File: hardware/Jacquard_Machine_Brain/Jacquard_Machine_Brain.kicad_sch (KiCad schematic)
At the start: 69 parts, among them J1 Terminal Block, J15 USB_A, J16 Wurth_RJ45_LED, J2 Conn_01x08, J3 JST-SH 01x04, J4 Conn_01x02, J5 Conn_01x02, SW1 SW_DIP_x02, SW2 SW_MEC_5G, U1 R-78E5.0-1.0, U10 74AHCT1G125, U2 Teensy4.1, U3 74AHCT1G125, U4 74AHCT1G125, U5 74AHCT125, U6 AO4882, U7 74AHCT1G125, U8 74AHCT1G125, U9 PCA9306D

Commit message: sync
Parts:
- removed C6: 0.1uF, Capacitor_SMD:C_0402_1005Metric, symbol Device:C_Small
- removed JP1, JP2, JP5, JP6, JP7, JP8: SolderJumper_2_Bridged, Jumper:SolderJumper-2_P1.3mm_Bridged_RoundedPad1.0x1.5mm, symbol Jumper:SolderJumper_2_Bridged
- removed R12, R13: 4.7k, Resistor_SMD:R_0603_1608Metric, symbol Device:R_Small
- removed U5: 74AHCT125, Package_SO:TSSOP-14_4.4x5mm_P0.65mm, symbol 0_integrated_circuits:74AHCT125_Multi
- added JP1, JP2, JP5: SolderJumper_3_Bridged123, Jumper:SolderJumper-3_P1.3mm_Bridged123_RoundedPad1.0x1.5mm_NumberLabels, symbol Jumper:SolderJumper_3_Bridged123
- added R17, R18, R19, R20: 4.7k, Resistor_SMD:R_0603_1608Metric, symbol Device:R_Small
- C9: value 0.1uF -> 100pF; LCSC C1525 -> C1546; Link https://www.digikey.com/en/products/detail/samsung-electro-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 -> (none); Manu # CL05B104KO5NNNC -> 0402CG101J500NT; Manu. Samsung Electro-Mechanics -> FH (Guangdong Fenghua Advanced Tech)
- U9: LCSC (none) -> C2677369
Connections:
- net +3V3: now also JP1.2 (C), JP2.2 (C)
- net +5V: now also JP5.2 (C); no longer R15.1, R16.1
- net GATE_1: now also R4.1
- net GATE_2: now also R5.1
- net SCL_0_3.3V: now also R19.2
- net SCL_0_5V: now also R15.2
- net SCL_1: now also R18.2
- net SDA_0_3.3V: now also R20.2
- net SDA_0_5V: now also R16.2
- net SDA_1: now also R17.2
- new net: JP1.1 (A), R18.1
- new net: JP1.3 (B), R17.1
- new net: JP2.1 (A), R20.1
- new net: JP2.3 (B), R19.1
- new net: JP5.1 (A), R16.1
- new net: JP5.3 (B), R15.1
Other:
- note added: "3.3V to 5V LEVEL CONVERSION FOR SHIFT REGISTER DRIVE"
- note added: "DUAL MOSFET SWITCHES"
- note added: "GP CONTROLS"
- note added: "MOSFET GATE DRIVE"
- note added: "TEENSY 4.1"
- moved on the sheet: C10, C11, C12, C3, C4, C5, C7, C8, C9, D2, D3, D4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

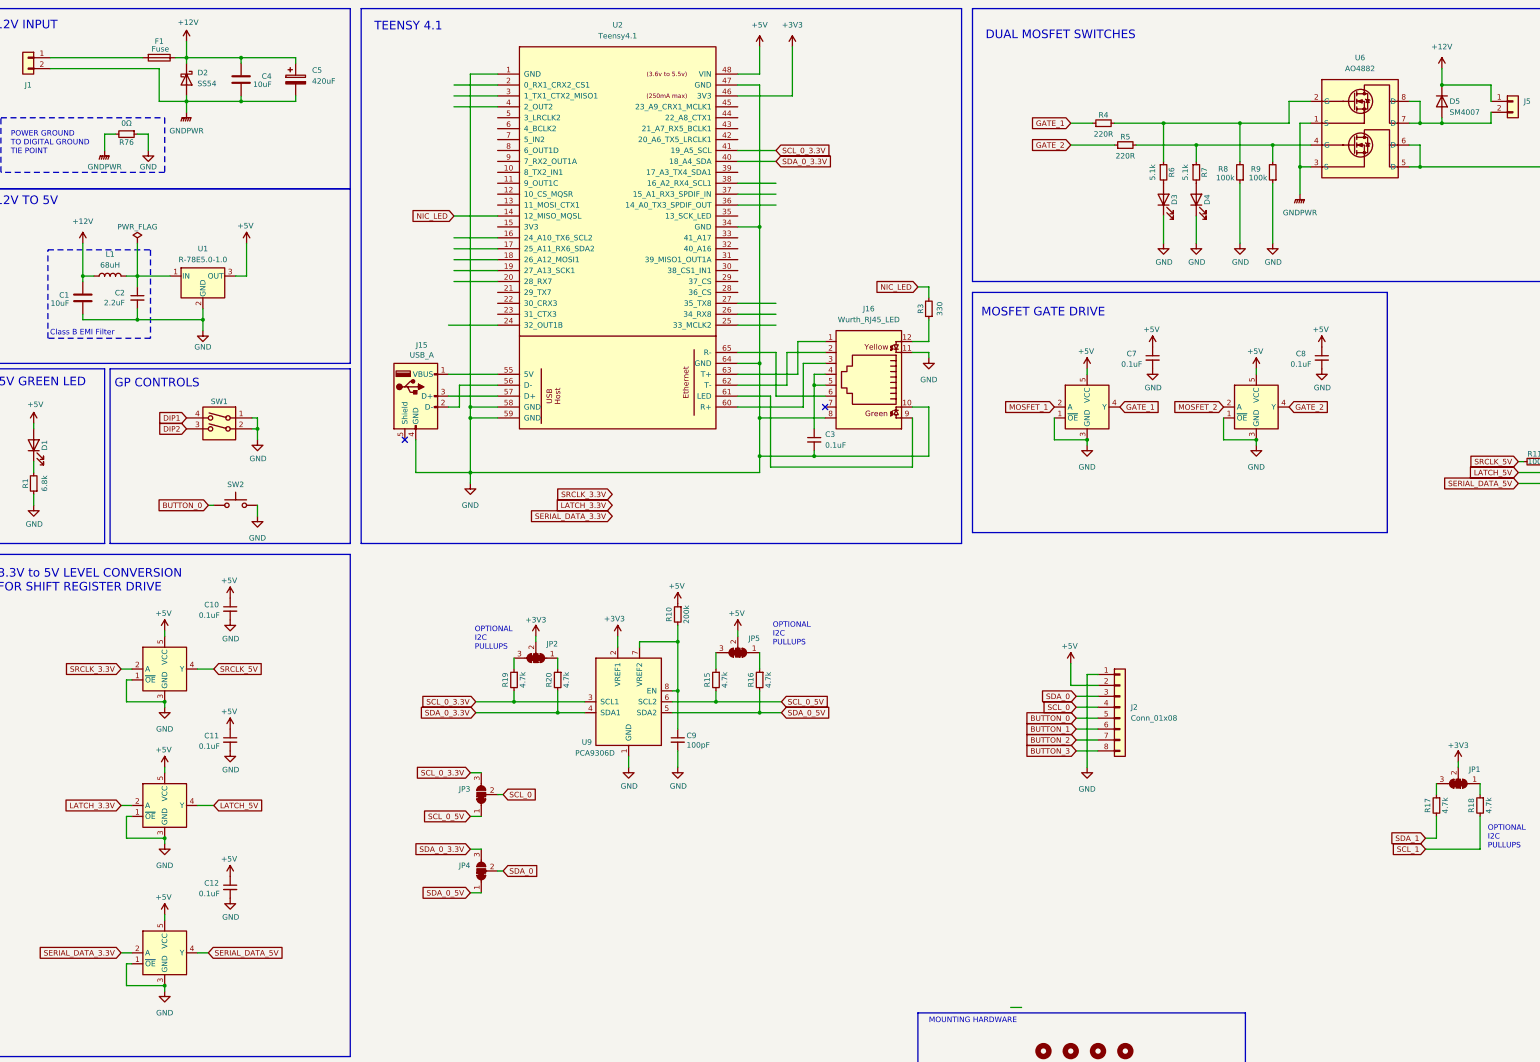
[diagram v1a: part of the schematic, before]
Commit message: Progress check
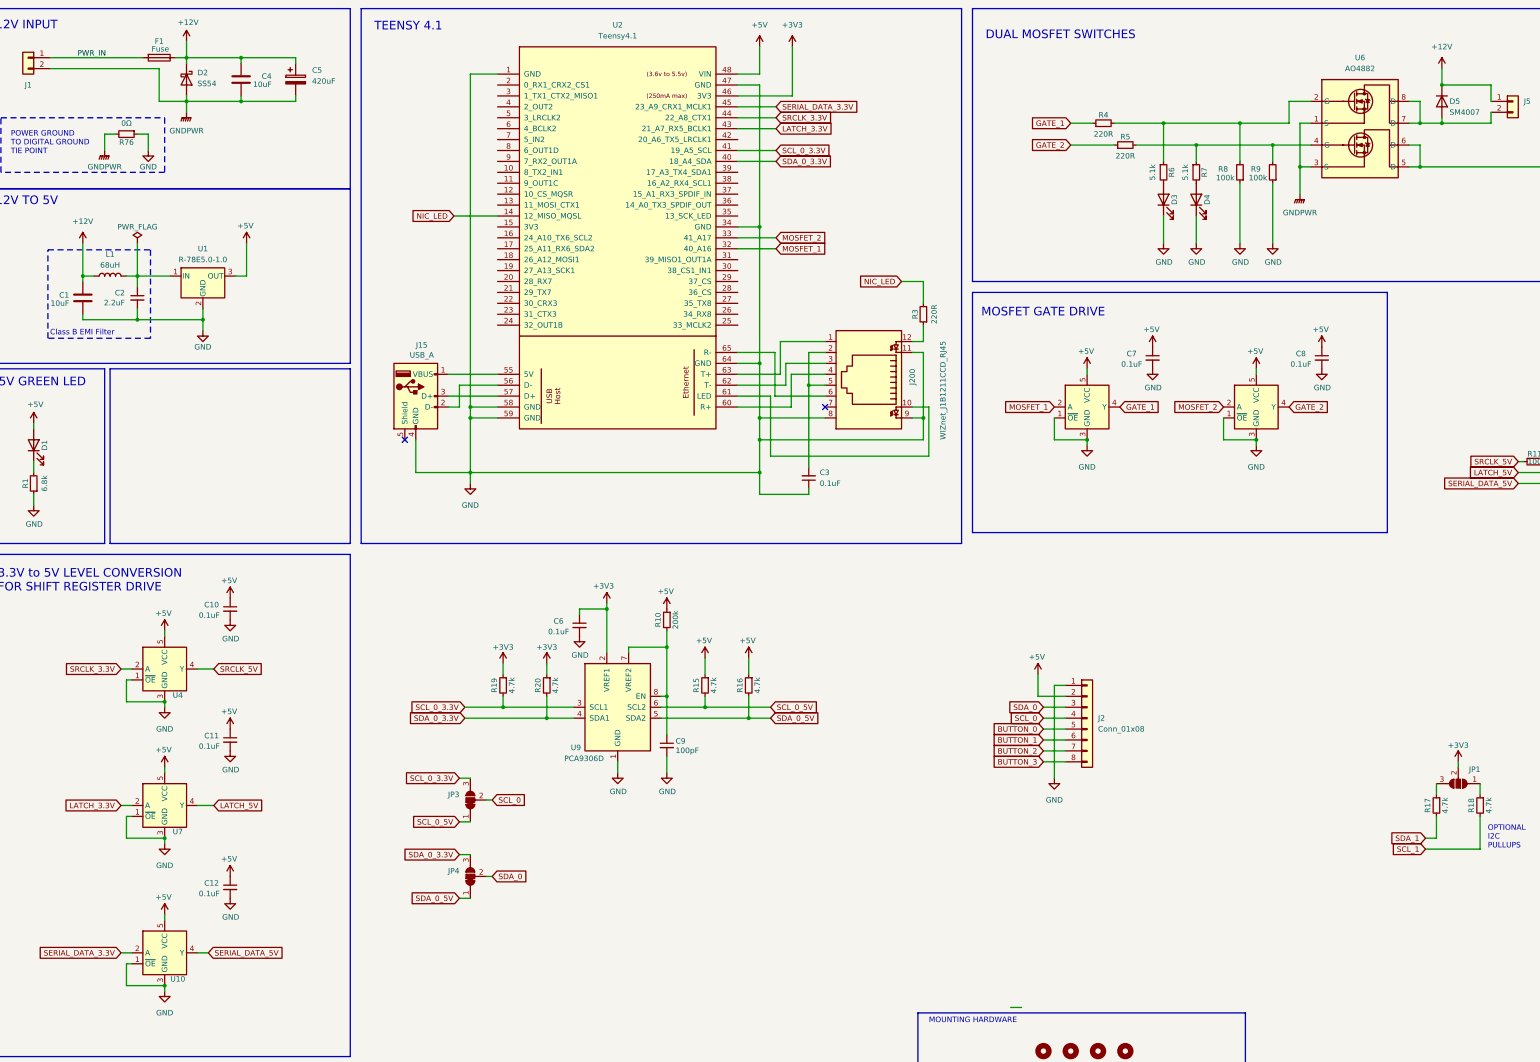
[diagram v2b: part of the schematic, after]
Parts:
- removed J16: Wurth_RJ45_LED, 0_connector:Wurth_7499010211A_RJ45, symbol 0_connector:Wurth_RJ45_LED
- removed JP2, JP5: SolderJumper_3_Bridged123, Jumper:SolderJumper-3_P1.3mm_Bridged123_RoundedPad1.0x1.5mm_NumberLabels, symbol Jumper:SolderJumper_3_Bridged123
- removed SW1: SW_DIP_x02, Button_Switch_THT:SW_DIP_SPSTx02_Slide_9.78x7.26mm_W7.62mm_P2.54mm, symbol Switch:SW_DIP_x02
- removed SW2: SW_MEC_5G, Button_Switch_THT:SW_TH_Tactile_Omron_B3F-100x, symbol Switch:SW_MEC_5G
- added C6: 0.1uF, Capacitor_SMD:C_0402_1005Metric, symbol Device:C_Small
- added J200: WIZnet_J1B1211CCD_RJ45, 0_connector:WIZnet_J1B1211CCD_RJ45, symbol 0_connector:WIZnet_J1B1211CCD_RJ45
- C3: footprint Capacitor_SMD:C_0805_2012Metric_Pad1.18x1.45mm_HandSolder -> Capacitor_SMD:C_0805_2012Metric; Digikey P/N (none) -> 311-1140-1-ND; Digikey Page (none) -> https://www.digikey.com/en/products/detail/yageo/CC0805KRX7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; LCSC (none) -> C49678; Link https://www.digikey.com/en/products/detail/samsung-electro-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 -> (none); Manu # CL21B104KBCNNNC -> CC0805KRX7R9BB104; Manu. Samsung Electro-Mechanics -> YAGEO
- F1: LCSC - -> C151075
- J1: LCSC - -> C89123
- J15: LCSC (none) -> C5815125
- JP1: footprint Jumper:SolderJumper-3_P1.3mm_Bridged123_RoundedPad1.0x1.5mm_NumberLabels -> Jumper:SolderJumper-3_P1.3mm_Open_RoundedPad1.0x1.5mm; symbol Jumper:SolderJumper_3_Bridged123 -> Jumper:SolderJumper_3_Open
- R3: value 330 -> 220R; footprint Resistor_SMD:R_0805_2012Metric_Pad1.20x1.40mm_HandSolder -> Resistor_SMD:R_0805_2012Metric; Digikey P/N (none) -> 311-220CRCT-ND; Digikey Page (none) -> https://www.digikey.com/en/products/detail/yageo/RC0805FR-0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; LCSC (none) -> C17557; Link https://mou.sr/4eszNXH -> (none); Manu # ERJ-P06J331V -> RC0805FR-07220RL; Manu. Panasonic -> YAGEO
- U1: LCSC - -> C22371890
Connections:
- net +3V3: now also R19.1, R20.1, C6.1
- net +5V: now also R15.1, R16.1
- net GND: now also C3.1, C6.2, J200.11, J200.8, J200.9; no longer C3.2
- net LATCH_3.3V: now also U2.43 (21_A7_RX5_BCLK1)
- net MOSFET_1: now also U2.32 (40_A16)
- net MOSFET_2: now also U2.33 (41_A17)
- net SERIAL_DATA_3.3V: now also U2.45 (23_A9_CRX1_MCLK1)
- net SRCLK_3.3V: now also U2.44 (22_A8_CTX1)
- net at R3.1: now also J200.12
- net at U2.63 (T+): now also J200.1
- net at U2.62 (T-): now also J200.3
- net at U2.60 (R+): now also J200.4
- net at U2.65 (R-): now also J200.6
- net at U2.61 (LED): now also J200.10
- net PWR_IN: now reaches F1.2, J1.1 (Pin_1)
- new net: C3.2, J200.2, J200.5
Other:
- note removed: "GP CONTROLS"
- moved on the sheet: C9, J2, JP3, JP4, R10, R15, R16, R19, R20, U9

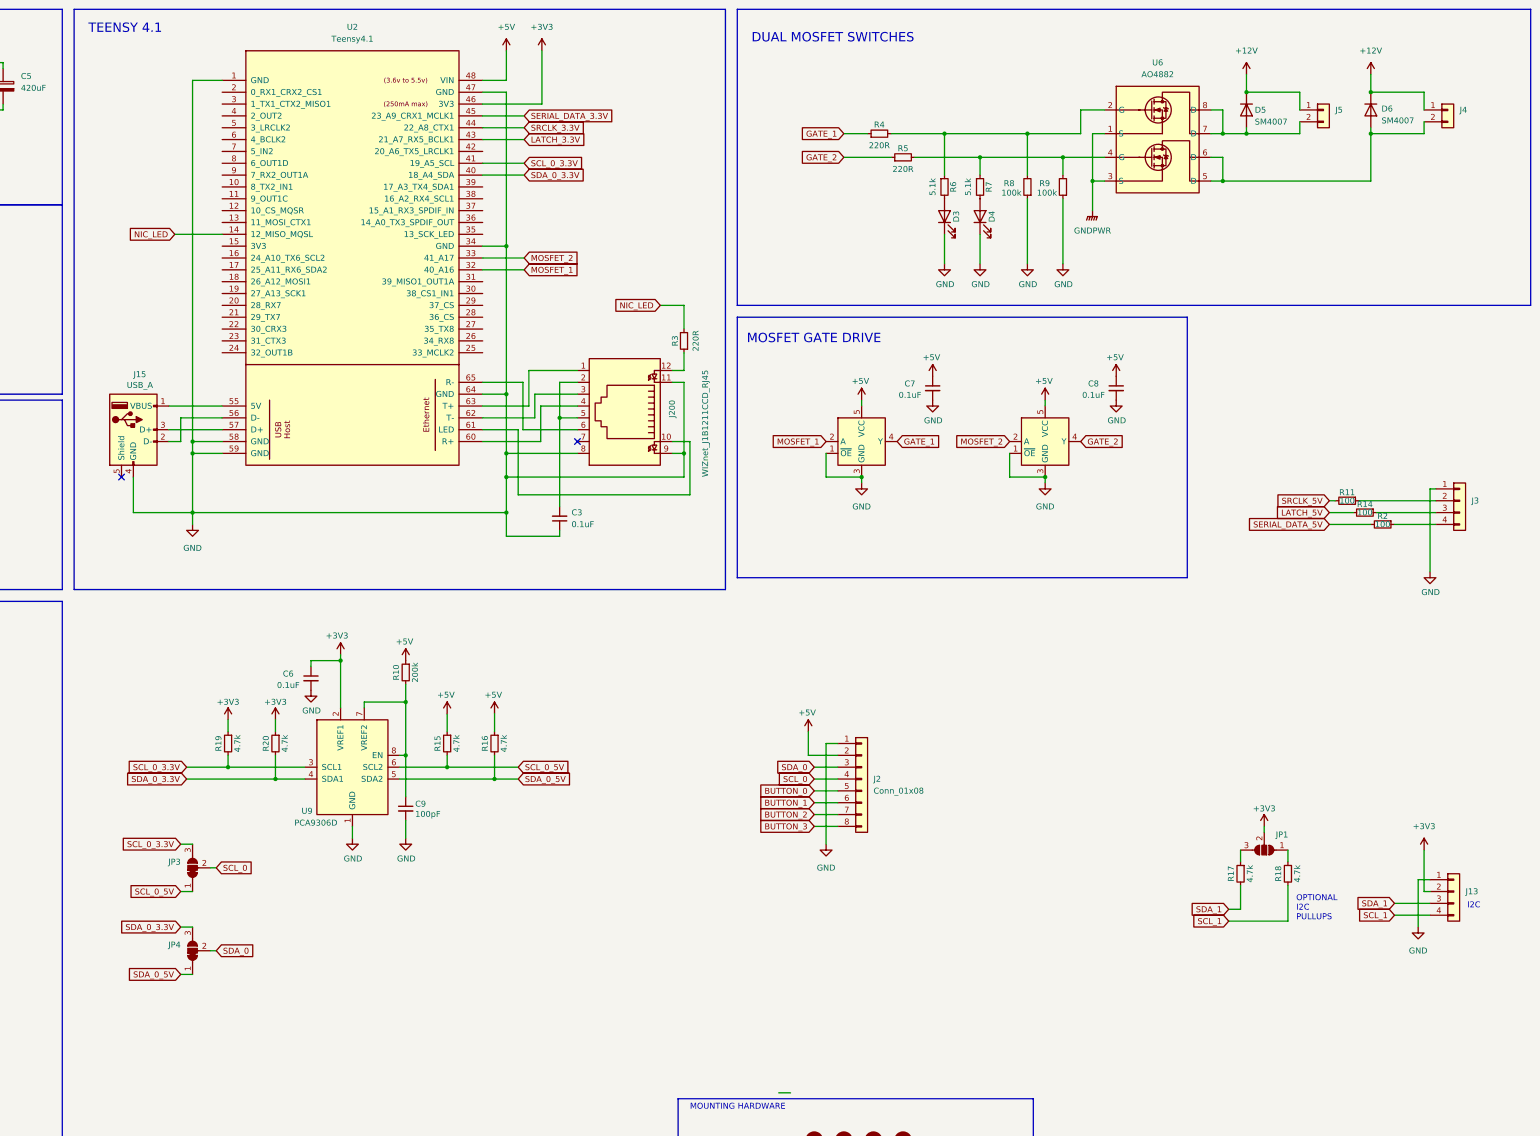
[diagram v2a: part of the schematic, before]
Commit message: sync
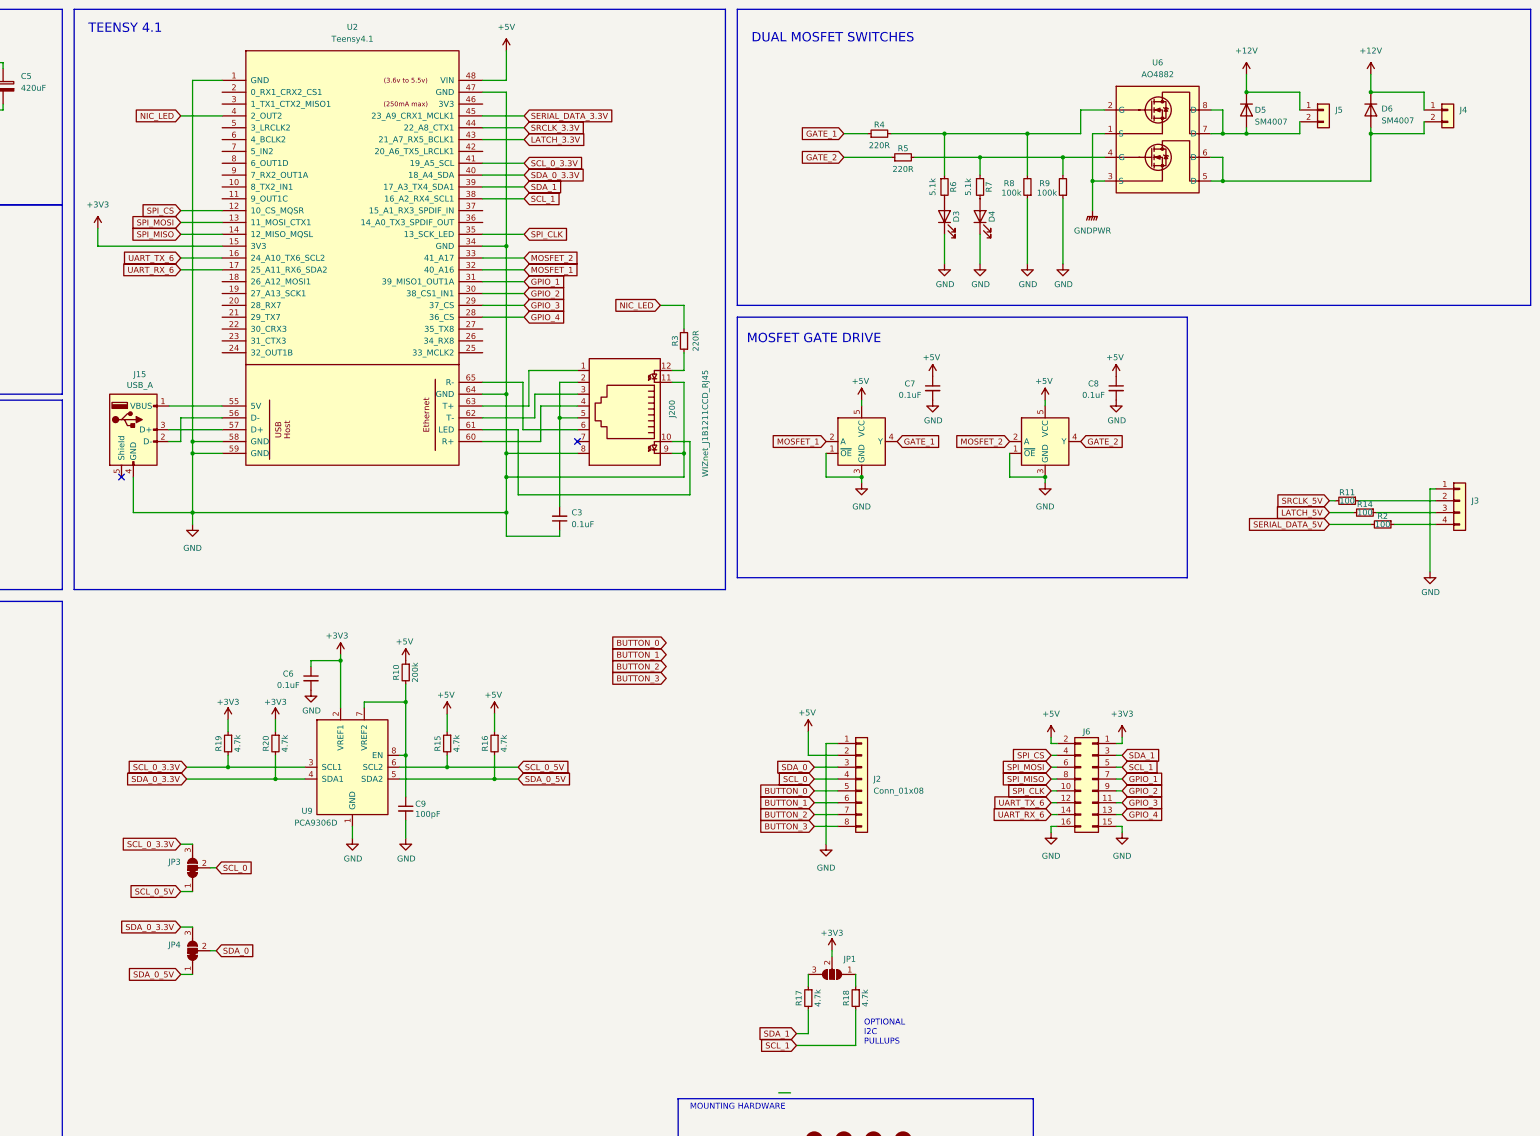
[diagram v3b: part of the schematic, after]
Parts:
- removed J13: ~, Connector_PinSocket_2.54mm:PinSocket_1x04_P2.54mm_Vertical, symbol 0_connector:Molex Micro-Fit 4pos
- added J6: Conn_02x08_Odd_Even, Connector_PinSocket_2.54mm:PinSocket_2x08_P2.54mm_Vertical, symbol Connector_Generic:Conn_02x08_Odd_Even
- J2: LCSC (none) -> C42431840
- J4, J5: LCSC (none) -> C7499322
- R10: LCSC (none) -> C25764
- U2: LCSC (none) -> C41376163
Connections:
- net +3V3: now also U2.15 (3V3), J6.1 (Pin_1); no longer U2.46 (3V3)
- net +5V: now also J6.2 (Pin_2)
- net GND: now also J6.15 (Pin_15), J6.16 (Pin_16)
- net NIC_LED: now also U2.4 (2_OUT2); no longer U2.14 (12_MISO_MQSL)
- net SCL_1: now also U2.38 (16_A2_RX4_SCL1), J6.5 (Pin_5)
- net SDA_1: now also U2.39 (17_A3_TX4_SDA1), J6.3 (Pin_3)
- net SPI_CS: now reaches U2.12 (10_CS_MQSR)
- net SPI_CS: now also J6.4 (Pin_4)
- net SPI_MOSI: now reaches U2.13 (11_MOSI_CTX1)
- net SPI_MOSI: now also J6.6 (Pin_6)
- net UART_TX_6: now reaches U2.16 (24_A10_TX6_SCL2)
- net UART_TX_6: now also J6.12 (Pin_12)
- net UART_RX_6: now reaches U2.17 (25_A11_RX6_SDA2)
- net UART_RX_6: now also J6.14 (Pin_14)
- net GPIO_4: now reaches U2.28 (36_CS)
- net GPIO_4: now also J6.13 (Pin_13)
- net GPIO_3: now reaches U2.29 (37_CS)
- net GPIO_3: now also J6.11 (Pin_11)
- net GPIO_2: now reaches U2.30 (38_CS1_IN1)
- net GPIO_2: now also J6.9 (Pin_9)
- net GPIO_1: now reaches U2.31 (39_MISO1_OUT1A)
- net GPIO_1: now also J6.7 (Pin_7)
- net SPI_CLK: now reaches U2.35 (13_SCK_LED)
- net SPI_CLK: now also J6.10 (Pin_10)
- new net SPI_MISO: J6.8 (Pin_8), U2.14 (12_MISO_MQSL)
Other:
- note removed: "I2C"
- moved on the sheet: JP1, R17, R18
